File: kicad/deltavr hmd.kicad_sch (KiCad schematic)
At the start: 10 parts, among them J1 Conn_02x07_Top_Bottom, U1 LSM6DSVTR, U2 nice_nano

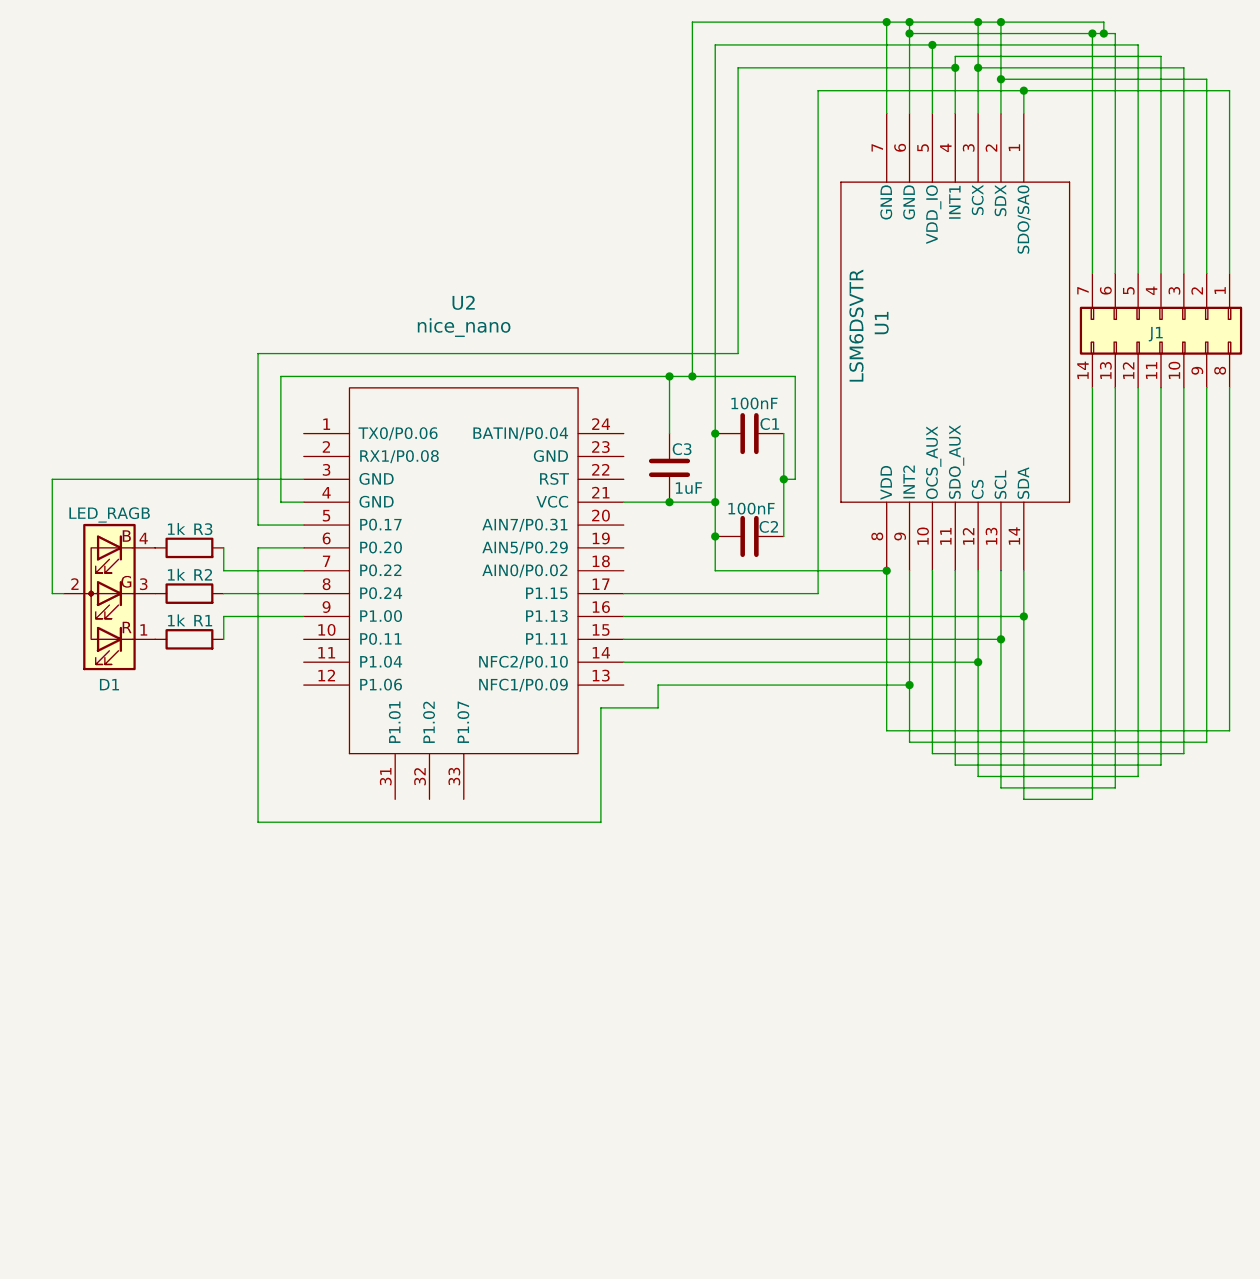
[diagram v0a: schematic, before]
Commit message: kicad files after save for final pcb for hmd module
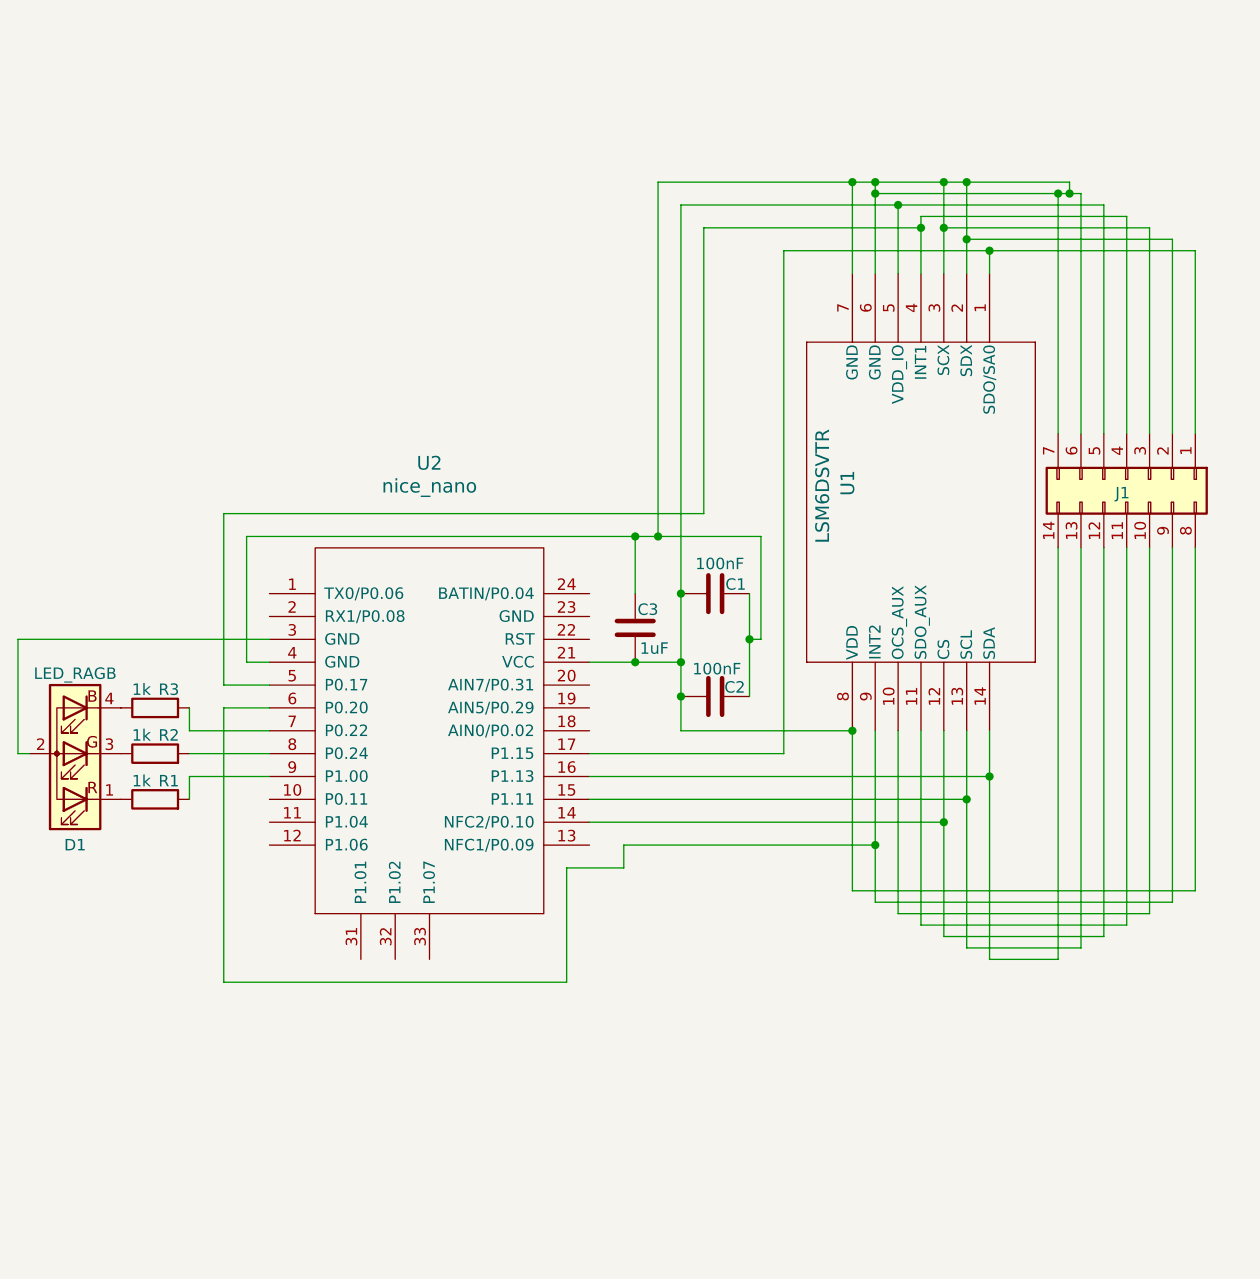
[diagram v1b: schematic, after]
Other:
- moved on the sheet: C1, C2, C3, D1, J1, R1, R2, R3, U1, U2

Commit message: hmd and controller done officially
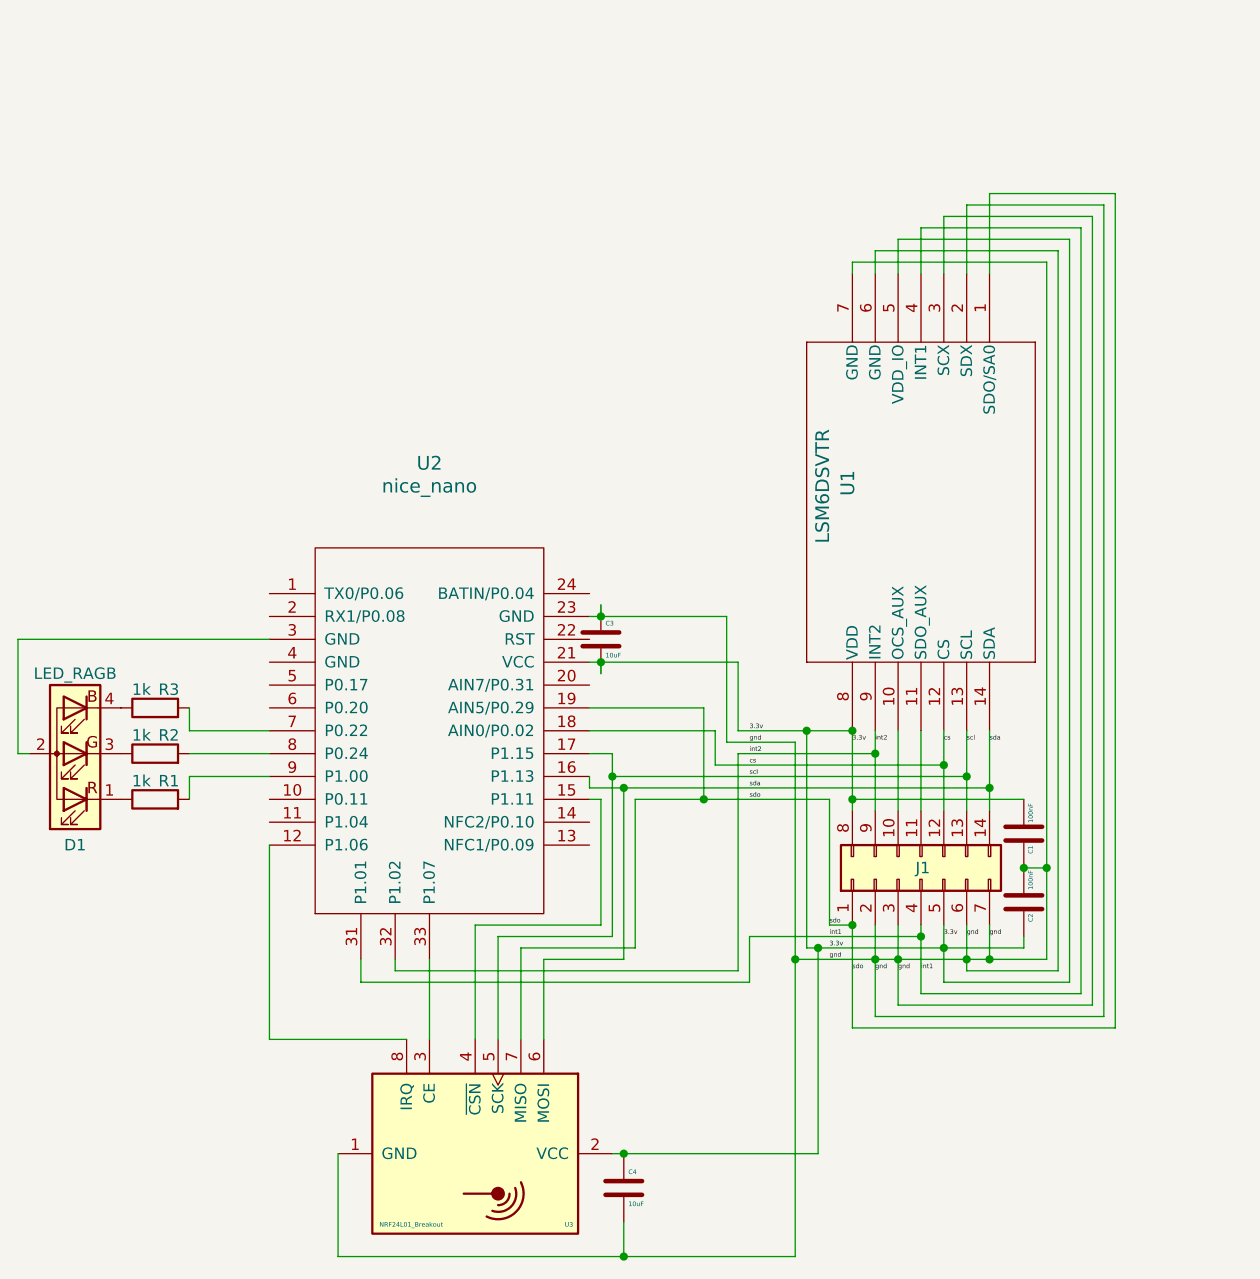
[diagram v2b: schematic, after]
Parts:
- added C4: 10uF, Capacitor_SMD:C_0603_1608Metric_Pad1.08x0.95mm_HandSolder, symbol Device:C
- added U3: NRF24L01_Breakout, RF_Module:nRF24L01_Breakout, symbol RF:NRF24L01_Breakout
- C3: value 1uF -> 10uF
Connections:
- net 3.3v: now reaches C3.1, J1.5 (Pin_5), J1.8 (Pin_8), U1.5 (VDD_IO), U1.8 (VDD), U2.21 (VCC)
- net 3.3v: now also C1.2, C2.1, C4.2, U3.2 (VCC); no longer C1.1, C2.2
- net gnd: now reaches C3.2, J1.2 (Pin_2), J1.3 (Pin_3), J1.6 (Pin_6), J1.7 (Pin_7), U1.2 (SDX), U1.3 (SCX), U1.6 (GND), U1.7 (GND)
- net gnd: now also C1.1, C2.2, U2.23 (GND), C4.1, U3.1 (GND); no longer C1.2, C2.1, U2.4 (GND)
- net sdo: now reaches J1.1 (Pin_1), U1.1 (SDO/SA0)
- net sdo: now also U2.19 (AIN5/P0.29), U3.7 (MISO); no longer U2.17 (P1.15)
- net cs: now reaches J1.12 (Pin_12), U1.12 (CS)
- net cs: now also U2.18 (AIN0/P0.02); no longer U2.14 (NFC2/P0.10)
- net scl: now reaches J1.13 (Pin_13), U1.13 (SCL)
- net scl: now also U2.17 (P1.15), U3.5 (SCK); no longer U2.15 (P1.11)
- net sda: now reaches J1.14 (Pin_14), U1.14 (SDA), U2.16 (P1.13)
- net sda: now also U3.6 (MOSI)
- net int1: now reaches J1.4 (Pin_4), U1.4 (INT1)
- net int1: now also U2.31 (P1.01); no longer U2.5 (P0.17)
- net int2: now reaches J1.9 (Pin_9), U1.9 (INT2)
- net int2: now also U2.32 (P1.02); no longer U2.6 (P0.20)
- net at U2.12 (P1.06): now also U3.8 (IRQ)
- net at U2.33 (P1.07): now also U3.3 (CE)
- new net: U2.15 (P1.11), U3.4 (~{CSN})
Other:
- moved on the sheet: C1, C2, C3, J1

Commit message: small chnages
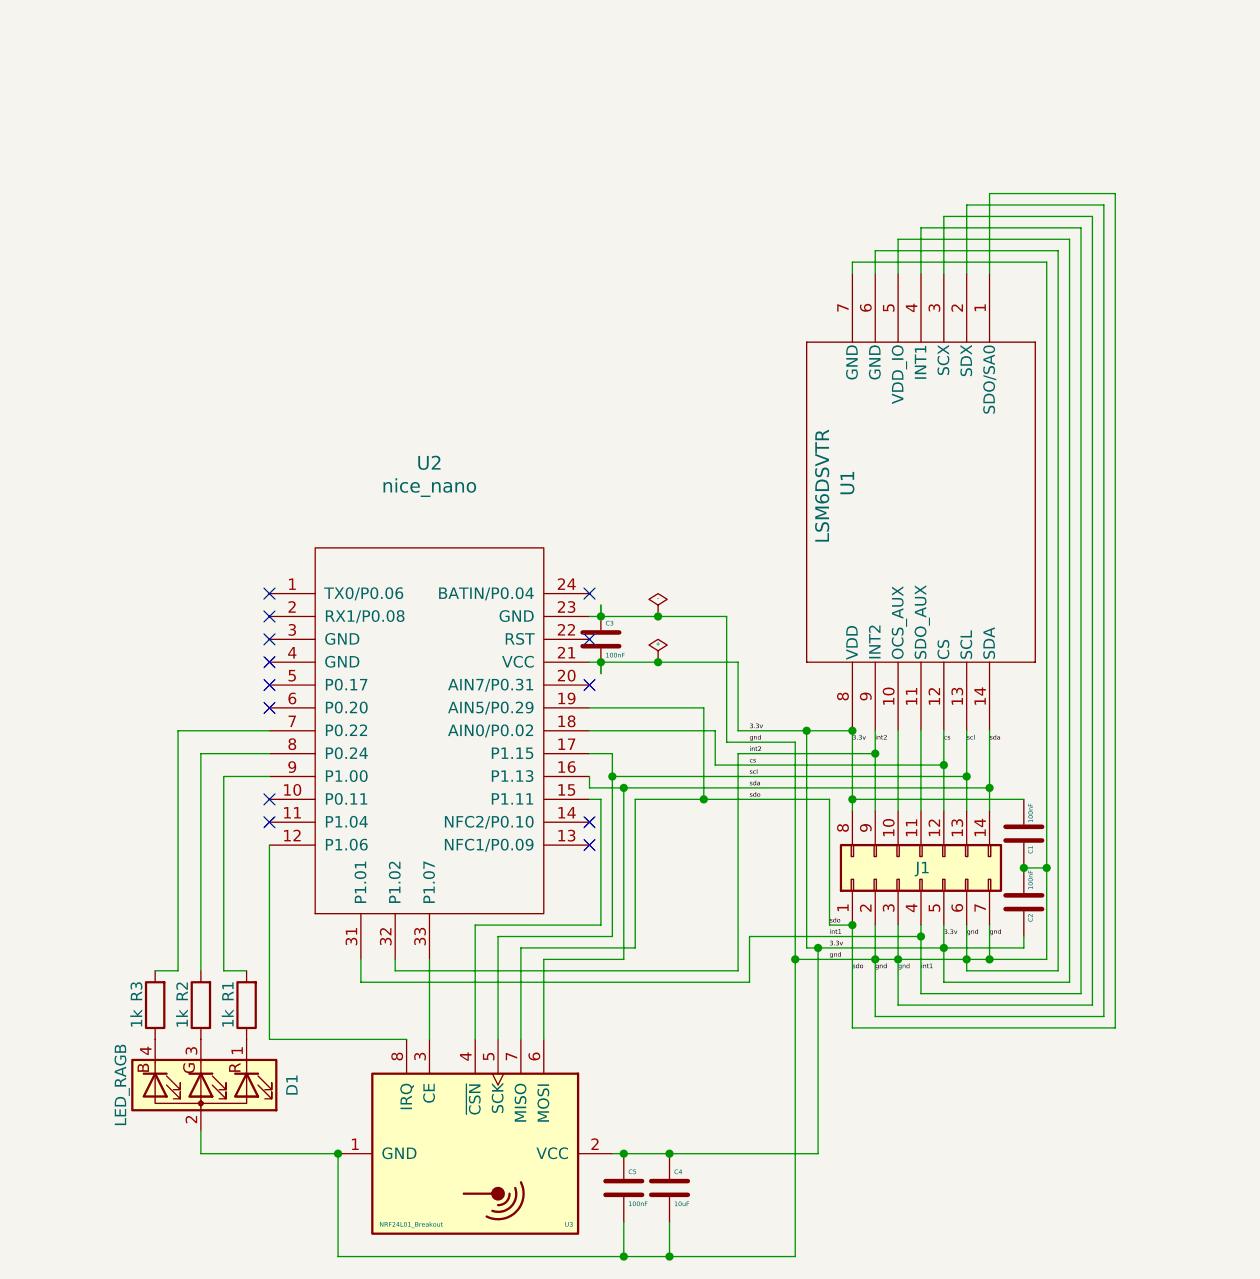
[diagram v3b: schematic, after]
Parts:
- added C5: 100nF, Capacitor_SMD:C_0603_1608Metric_Pad1.08x0.95mm_HandSolder, symbol Device:C
- C3: value 10uF -> 100nF
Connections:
- net 3.3v: now also C5.2
- net gnd: now also D1.2 (A), C5.1
- net at U2.3 (GND): no longer D1.2 (A)
- no-connect marks 0 -> 13
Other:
- moved on the sheet: C4, D1, R1, R2, R3
